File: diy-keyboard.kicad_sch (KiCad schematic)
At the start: 16 parts

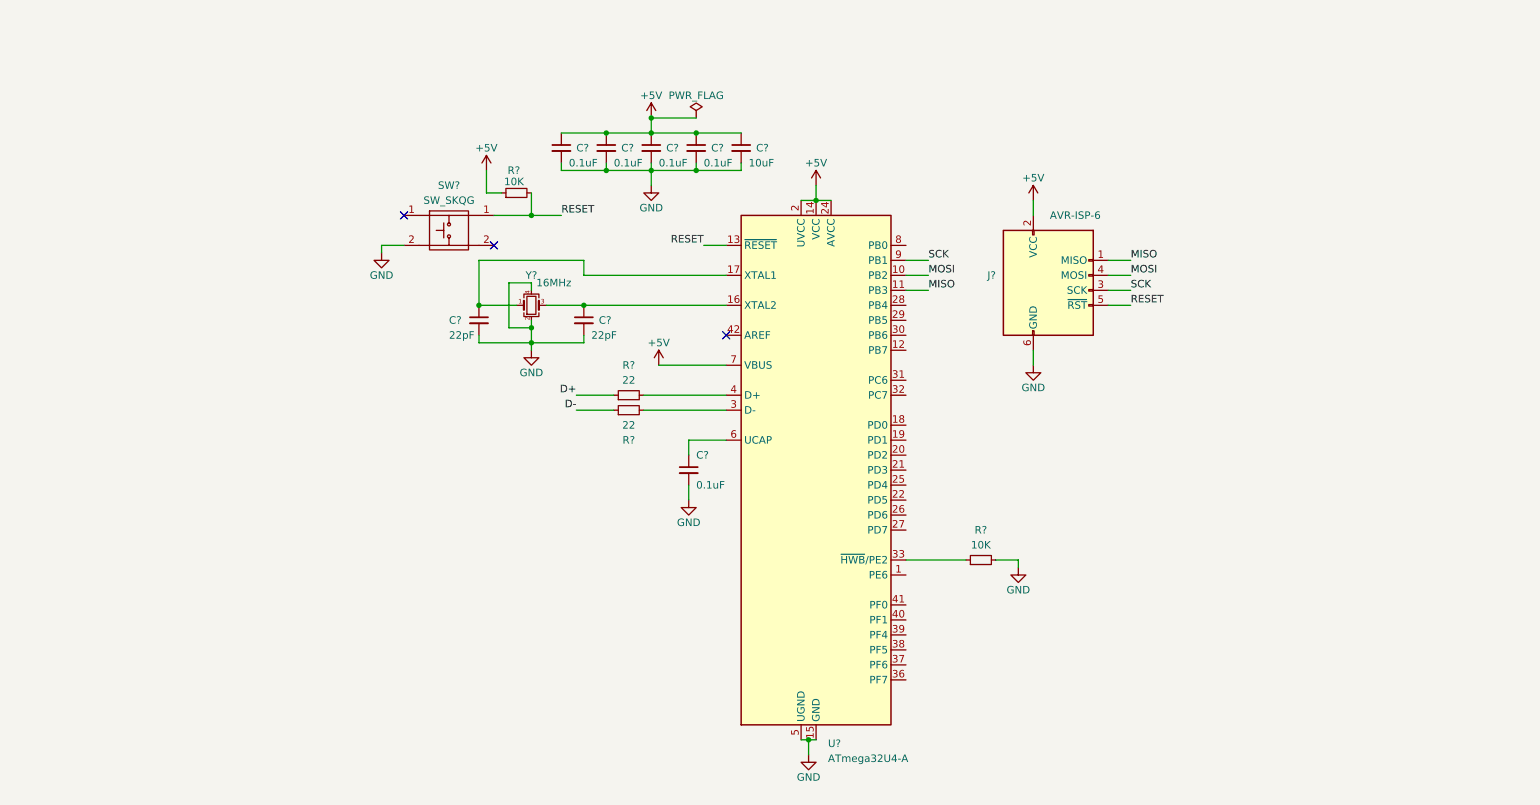
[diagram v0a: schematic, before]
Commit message: Update Library and schematic
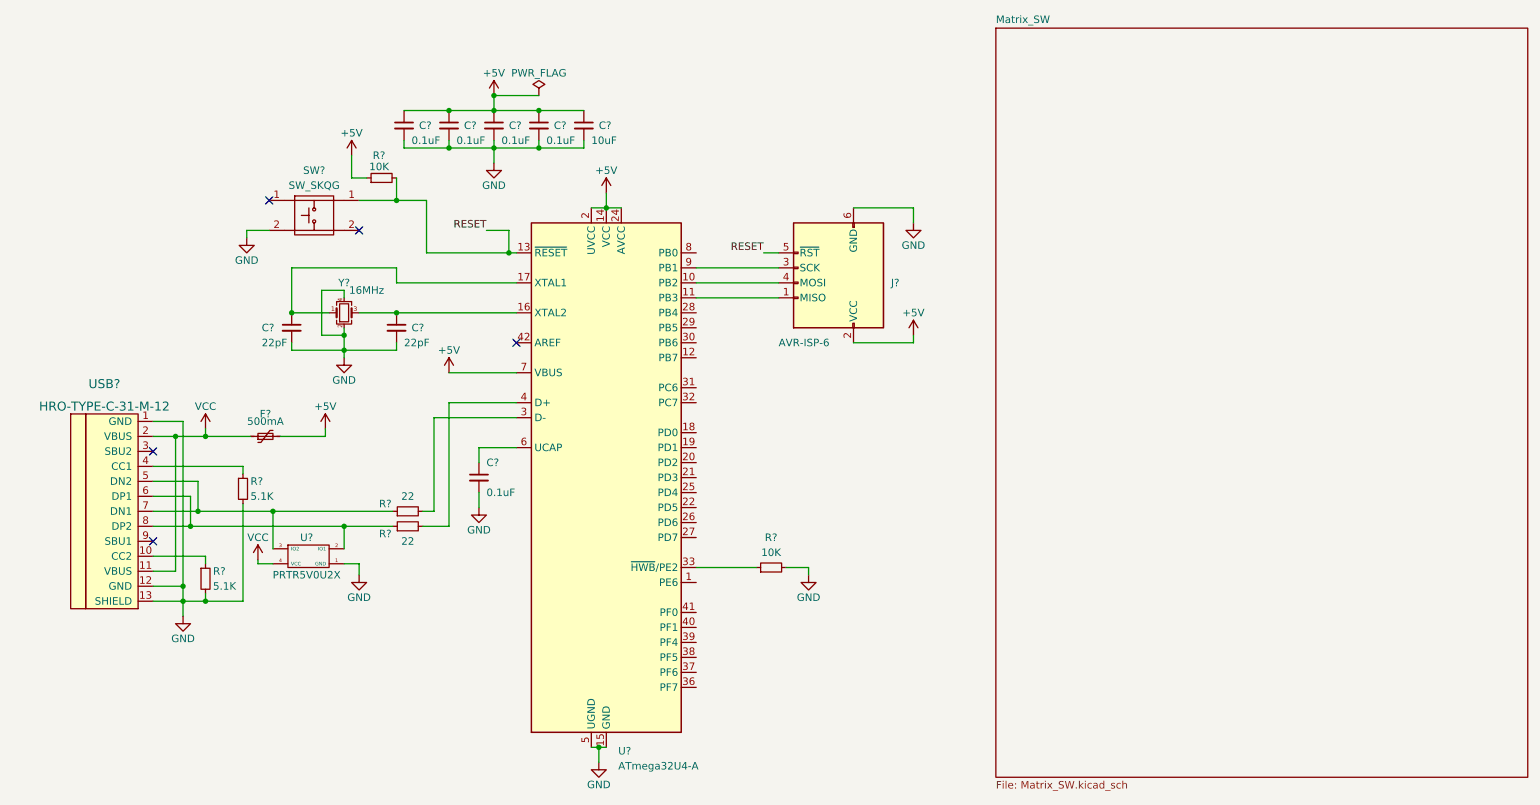
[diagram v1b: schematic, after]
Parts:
- added F?: 500mA, symbol Device:Polyfuse_Small
- added R? (x2): 5.1K, symbol Device:R_Small
- added U?: PRTR5V0U2X, Package_TO_SOT_SMD:SOT-143, symbol PWR_protection:PRTR5V0U2X
- added USB?: HRO-TYPE-C-31-M-12, symbol Type-C:HRO-TYPE-C-31-M-12
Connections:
- net +5V: now also F?.2
- net GND: now also R?.2, R?.2, U?.1 (GND), USB?.1 (GND), USB?.12 (GND), USB?.13 (SHIELD)
- net at R?.2: now also U?.3 (D-); no longer U?.4 (D+)
- net at R?.2: now also U?.4 (D+); no longer U?.3 (D-)
- net D+: no longer names the net of R?.1
- net D+: now also U?.3 (IO2), USB?.5 (DN2), USB?.7 (DN1)
- net D-: no longer names the net of R?.1
- net D-: now also U?.2 (IO1), USB?.6 (DP1), USB?.8 (DP2)
- net MISO: no longer names the net of J?.1 (MISO), U?.11 (PB3)
- net MOSI: no longer names the net of J?.4 (MOSI), U?.10 (PB2)
- net SCK: no longer names the net of J?.3 (SCK), U?.9 (PB1)
- new net: R?.1, USB?.10 (CC2)
- new net: R?.1, USB?.4 (CC1)
- new net VCC: F?.1, U?.4 (VCC), USB?.11 (VBUS), USB?.2 (VBUS)
- no-connect marks 3 -> 5
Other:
- added sheet Matrix_SW (Matrix_SW.kicad_sch)
- moved on the sheet: C?, J?, R?, SW?, U?, Y?
